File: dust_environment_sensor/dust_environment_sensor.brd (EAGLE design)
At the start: 70.8 x 68.7 mm, 36 parts, among them J1 3.6V Lithium C cell, U1 LTP5901, U2 LIS3DH, U3 SI7005, U4 TSL2560, U5 ATMEGA328P, X1 32.768KHz

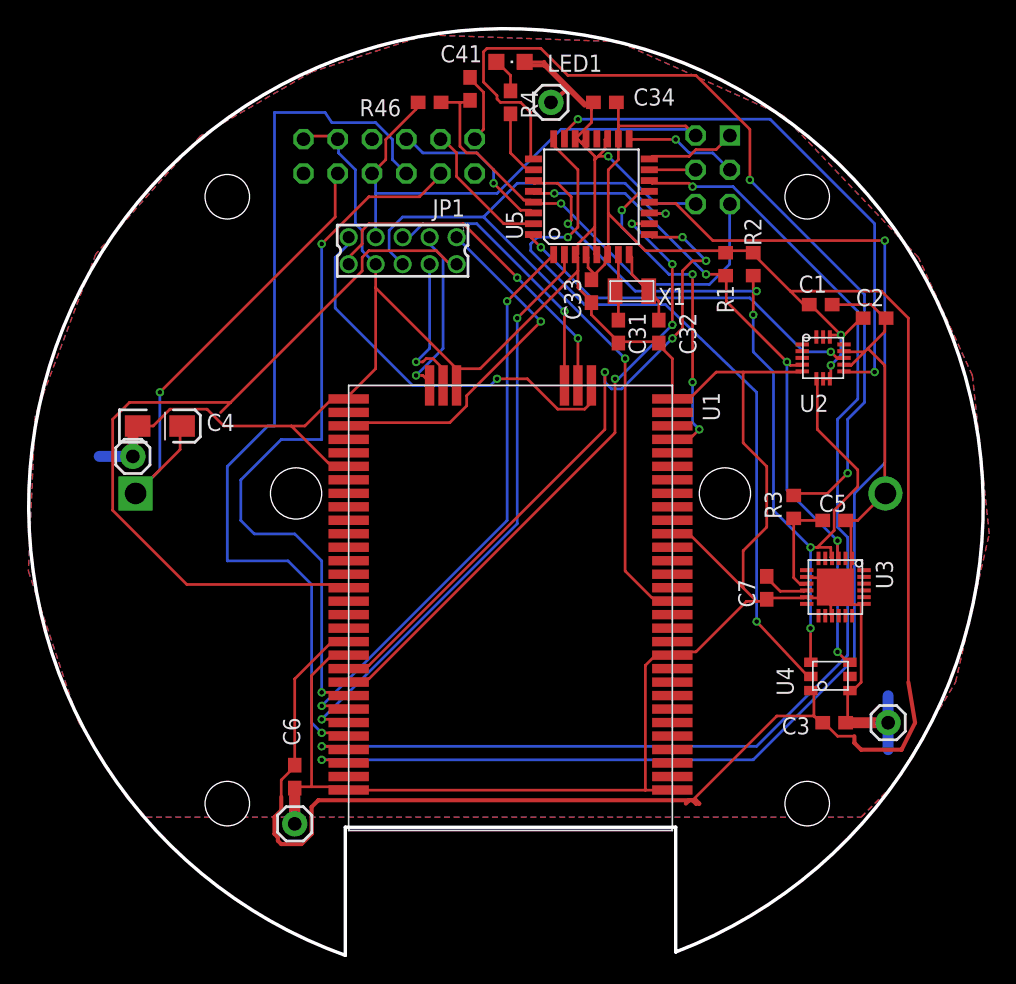
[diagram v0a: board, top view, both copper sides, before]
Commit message: Latest Powerstrip changes
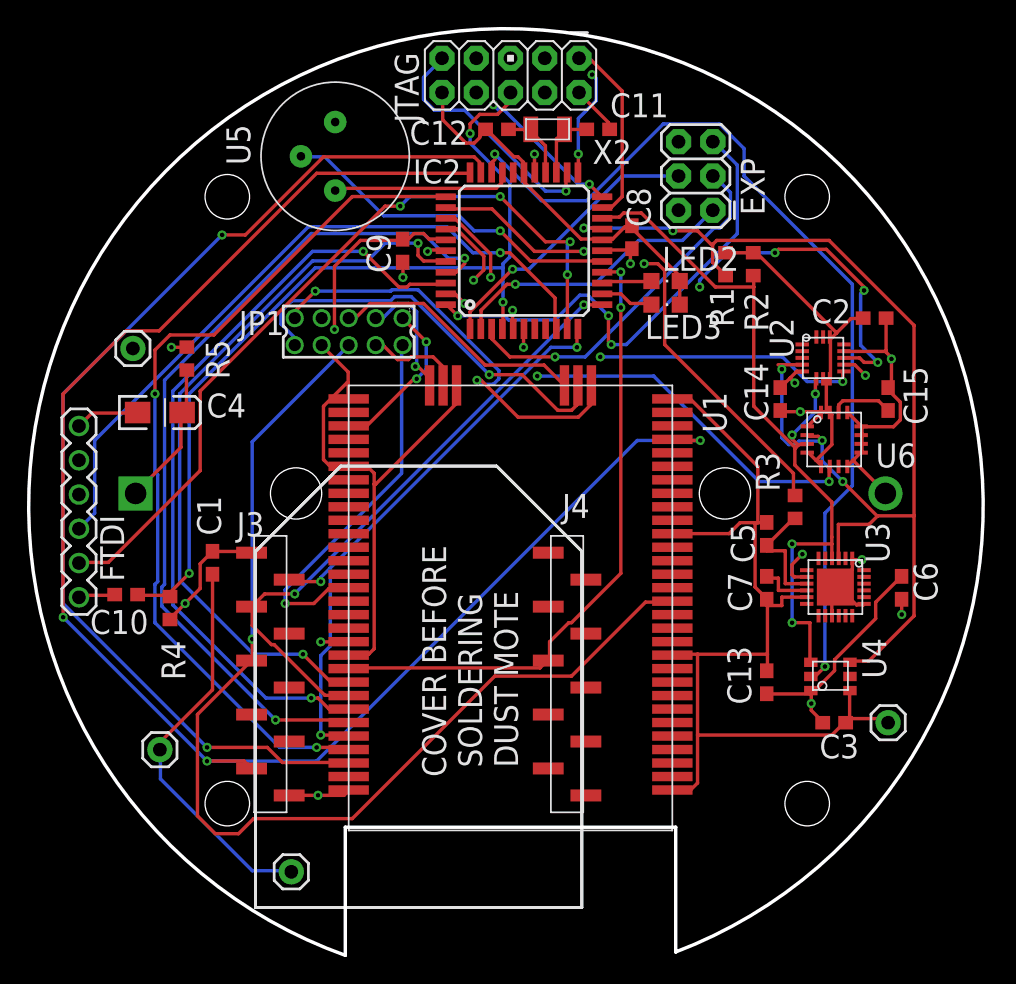
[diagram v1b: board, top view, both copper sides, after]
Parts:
- removed C31, C32: 22p, SparkFun:0603
- removed C33, C34, C41: .1u, SparkFun:0603
- removed JP2: AVR_SPI_PRG_6NS, SparkFun:2X3-NS
- removed JP3: .1" header, con-lstb:MA06-2
- removed LED1: RED, led:CHIPLED_0805
- removed R46: 10k, SparkFun:0603
- removed X1: 32.768KHz, WSNlib:ABS07
- added C10, C13, C15, C8, C9: 100n, rcl:C0603
- added C11, C12: TODO, rcl:C0603
- added C14: 10u, rcl:C0603
- added IC2: ATMEGA644A, atmel:TQFP44
- added J2: EXP, SparkFun-Connectors:2X3
- added J3: XBEE_1-10SMT, Cool_Electricity:XBEE_1-10_SMT
- added J4: XBEE_11-20SMT, Cool_Electricity:XBEE_11-20_SMT
- added JP8: (no value), custom:1X06
- added JP9: JTAG, SparkFun-Connectors:AVR_ICSP
- added LED2, LED3: (no value), led:CHIPLED_0805
- added R5: 0R, resistor:R0603
- added U6: L3GD20, Cool_Electricity:LGA16_4X4_ST
- added X2: 32.768KHz, WSNlib:ABS07
- R4: value 120 -> 10k; device SparkFun:0603 -> resistor:R0603
- U5: value ATMEGA328P -> AMN41121; device SparkFun:TQFP32-08 -> Cool_Electricity:AMN41121
- moved JP7 56.1 mm to (9.00, 17.0)
- moved C1 49.0 mm to (12.9, 30.9), turned to 270 degrees
- moved C6 47.1 mm to (64.0, 29.0)
- moved R4 45.2 mm to (9.75, 27.5)
- moved U5 19.2 mm to (22.0, 61.0), turned to 0 degrees
- moved JP6 8.00 mm to (7.00, 46.8)
- moved JP1 7.21 mm to (23.0, 48.0)
- moved C5 5.10 mm to (54.0, 33.0), turned to 90 degrees
- moved JP5 3.57 mm to (18.7, 7.94)
- moved C4 1.00 mm to (9.00, 42.0)
- moved R3 0.10 mm to (56.1, 35.0)
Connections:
- removed net ATMEGA_RX: JP3.7, U5.30
- removed net ATMEGA_TX: JP3.9, U5.31
- removed net MISO: JP2.1, U5.16
- removed net MOSI: JP2.4, U5.15
- removed net N$4: C32.1, U5.8, X1.1
- removed net N$5: LED1.A, R4.1
- removed net SCLK: JP2.3, U5.17
- new net ATMEGA_TO_FTDI: IC2.10, JP8.5
- new net EXP_CSN: IC2.44, J2.5
- new net EXP_MISO: IC2.2, J2.1
- new net EXP_MOSI: IC2.1, J2.4
- new net EXP_SCK: IC2.3, J2.3
- new net FTDI_TO_ATMEGA: IC2.9, JP8.4
- new net GYRO_INT2: IC2.43, U6.6
- new net LED2: IC2.13, LED3.A
- new net N$6: C11.1, IC2.25, X2.2
- new net N$7: C12.1, IC2.26, X2.1
- new net PIR_OUT: IC2.16, U5.OUT
- new net PIR_VCC: IC2.30, U5.VDD
- new net TCK: IC2.21, JP9.1
- new net TDI: IC2.24, JP9.9
- new net TDO: IC2.23, JP9.3
- new net TMS: IC2.22, JP9.5
- net ACCEL_INT1: now also IC2.37; no longer U5.32
- net ACCEL_INT2: now also IC2.36; no longer U5.23
- net GND: now also C11.2, C12.2, C13.2, C14.2, C15.2, C8.1, C9.1, IC2.18, IC2.28, IC2.39, IC2.6, J2.6, J3.10, JP8.1, JP8.2, JP9.10, JP9.2, LED2.C, LED3.C, U5.GND, U6.10, U6.11, U6.12, U6.13, U6.8, U6.9; no longer C31.2, C32.2, C33.1, C34.1, JP2.6, JP3.1, JP3.3, LED1.C, U5.19, U5.21, U5.22, U5.3, U5.5
- net HUMID_VCC: now also IC2.35; no longer U5.25
- net I2C_SCL: now also IC2.19, U6.2; no longer U5.28
- net I2C_SDA: now also IC2.20, U6.3; no longer U5.27
- net LED1: now also IC2.14, LED2.A; no longer R4.2, U5.26
- net LIGHT_INT: now also IC2.31; no longer U5.24
- net MOTE_API_RX: now also IC2.12, J3.3; no longer JP3.10
- net MOTE_API_TX: now also IC2.11, J3.2; no longer JP3.8
- net MOTE_RADIO_INHIBIT: now also IC2.32; no longer U5.12
- net MOTE_RESETN: now also J3.5; no longer U5.11
- net MOTE_RX_CTSN: now also IC2.40; no longer U5.10
- net MOTE_RX_RTSN: now also IC2.15, J4.16; no longer U5.9
- net MOTE_SLEEPN: now also IC2.33, J3.9; no longer U5.13
- net MOTE_TIMEN: now also IC2.34; no longer U5.14
- net MOTE_TX_CTSN: now also IC2.41; no longer U5.2
- net MOTE_TX_RTSN: now also IC2.42; no longer U5.1
- net N$2: now also C15.1, U6.14; no longer C31.1, U5.7, X1.2
- net RST: now also C10.1, IC2.4, JP9.6, R4.1; no longer C41.1, JP2.5, R46.1, U5.29
- net RTS#: now also C10.2, JP8.6; no longer C41.2, JP3.11
- net VBATT: now also R5.2; no longer JP3.4
- net VCC: now also C13.1, C14.1, C8.2, C9.2, IC2.17, IC2.27, IC2.38, IC2.5, J2.2, J3.1, JP9.4, R4.2, R5.1, U6.1, U6.15, U6.16, U6.4, U6.5; no longer C33.2, C34.2, JP2.2, JP3.6, R46.2, U5.18, U5.4, U5.6
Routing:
- net VCC: track 204.4 -> 83.8 mm, vias 2 -> 9
- net MOTE_SLEEPN: track 24.8 -> 120.7 mm, vias 4 -> 3
- net GND: track 296.7 -> 231.7 mm, vias 1 -> 10
- net ATMEGA_TO_FTDI: track 0.00 -> 59.1 mm, vias 0 -> 4
- net FTDI_TO_ATMEGA: track 0.00 -> 52.3 mm, vias 0 -> 1
- net EXP_CSN: track 0.00 -> 36.5 mm, vias 0 -> 3
- net GYRO_INT2: track 0.00 -> 35.4 mm, vias 0 -> 3
- net I2C_SCL: track 52.0 -> 87.1 mm
- net FLASH_P_ENN: track 59.5 -> 28.0 mm, vias 0 -> 1
- net RST: track 34.9 -> 66.3 mm, vias 1 -> 3
- net HUMID_VCC: track 67.0 -> 38.9 mm
- net EXP_SCK: track 0.00 -> 26.9 mm, vias 0 -> 1
- net VBATT: track 36.5 -> 10.7 mm, vias 1 -> 0
- net PIR_OUT: track 0.00 -> 25.6 mm, vias 0 -> 1
- net MOTE_TIMEN: track 89.9 -> 64.9 mm
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- added copper zone on layer 15, net GND
- added copper zone on layer 2, net VCC
- removed copper zone on layer 16, net GND
- removed copper zone on layer 1, net VCC
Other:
- board text added: "COVER BEFORE SOLDERING DUST MOTE"
- board text added: "Dust Sensor PCB Kevin Weekly"
- board text added: "EXP"
- board text added: "FTDI"
- board text added: "JTAG"

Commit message: BOM Updates
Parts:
- C11, C12: value TODO -> 10p
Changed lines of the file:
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@@
 <attribute name="VALUE" x="34.746" y="69.794" size="0.4064" layer="27" font="vector"/>
 </element>
-<element name="C11" library="rcl" package="C0603" value="TODO" x="41.5" y="63" smashed="yes">
+<element name="C11" library="rcl" package="C0603" value="10p" x="41.5" y="63" smashed="yes">
 <attribute name="NAME" x="42.389" y="63.889" size="1.778" layer="25"/>
 <attribute name="VALUE" x="40.865" y="61.095" size="1.27" layer="27"/>
 </element>
-<element name="C12" library="rcl" package="C0603" value="TODO" x="34" y="63" smashed="yes" rot="R180">
+<element name="C12" library="rcl" package="C0603" value="10p" x="34" y="63" smashed="yes" rot="R180">
 <attribute name="NAME" x="31.841" y="63.635" size="1.778" layer="25" rot="R180"/>
 <attribute name="VALUE" x="34.635" y="64.905" size="1.27" layer="27" rot="R180"/>
